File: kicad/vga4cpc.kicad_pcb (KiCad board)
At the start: 2 copper layers, 61.4 x 76.7 mm, 39 parts, among them J1 VGA socket, J2 CPC video port, SW1 VFreq sw, SW2 reset, U1 Pico

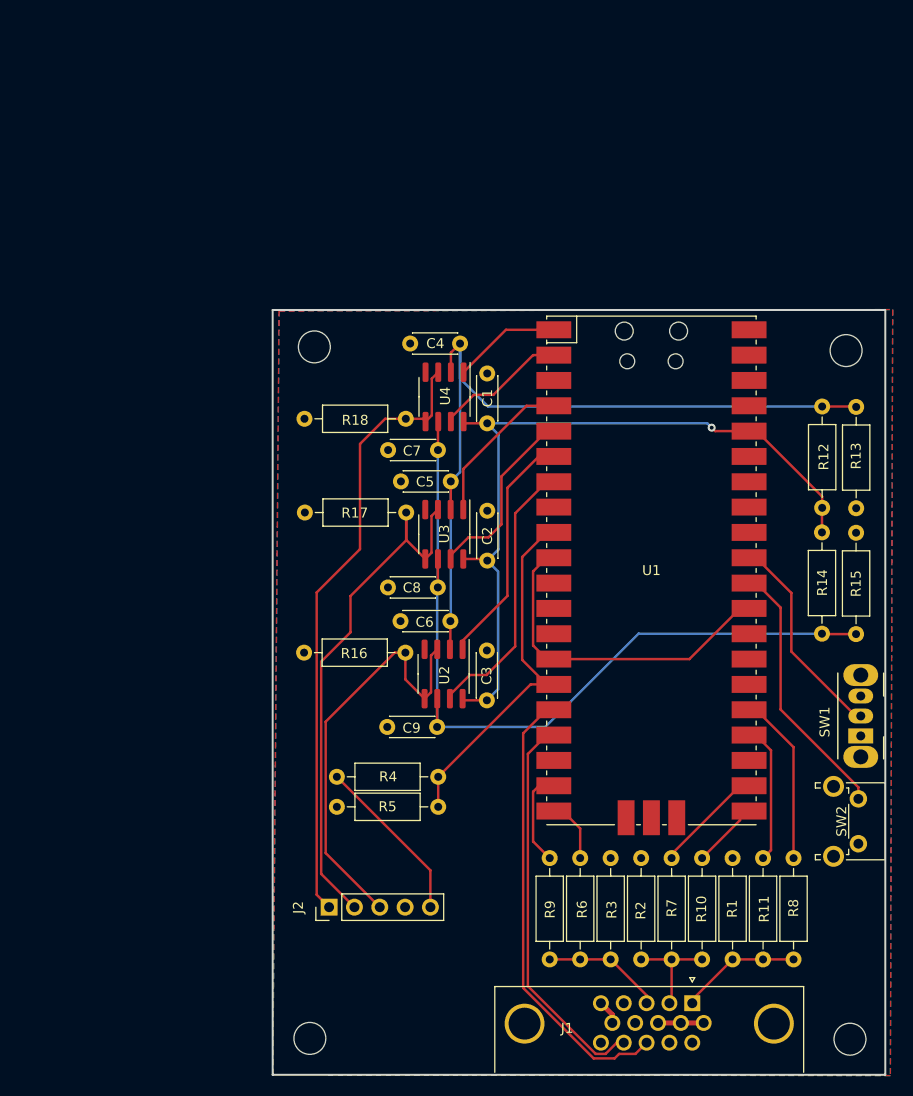
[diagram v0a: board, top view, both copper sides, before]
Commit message: Refactored
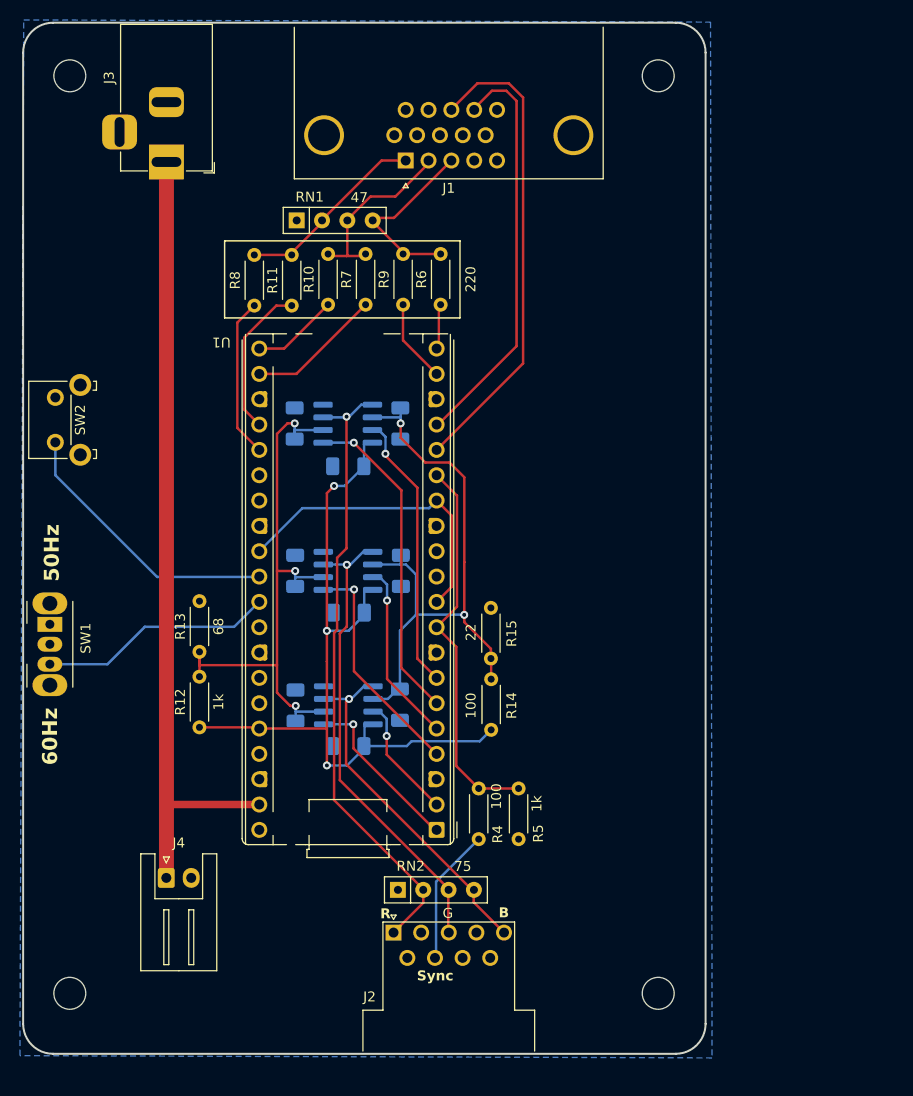
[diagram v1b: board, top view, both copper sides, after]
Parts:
- removed R1, R2, R3: 47, Resistor_THT:R_Axial_DIN0207_L6.3mm_D2.5mm_P10.16mm_Horizontal
- removed R16, R17, R18: 75, Resistor_THT:R_Axial_DIN0207_L6.3mm_D2.5mm_P10.16mm_Horizontal
- added J3: Barrel_Jack, Connector_BarrelJack:BarrelJack_Horizontal, F.Cu at (59.7, 36.6)
- added J4: Conn_01x02_Pin, Connector_JST:JST_XH_S2B-XH-A_1x02_P2.50mm_Horizontal, F.Cu at (59.7, 108.4)
- added RN1: 47, Resistor_THT:R_Array_SIP4, F.Cu at (72.8, 42.5)
- added RN2: 75, Resistor_THT:R_Array_SIP4, F.Cu at (82.9, 109.6)
- C1, C2, C3, C4, C5, C6, C7, C8, C9: footprint Capacitor_THT:C_Disc_D4.3mm_W1.9mm_P5.00mm -> Capacitor_SMD:C_1206_3216Metric_Pad1.33x1.80mm_HandSolder; moved to B.Cu
- J1: footprint Connector_Dsub:DSUB-15-HD_Female_Horizontal_P2.29x1.98mm_EdgePinOffset3.03mm_Housed_MountingHolesOffset4.94mm -> Connector_Dsub:DSUB-15-HD_Socket_Horizontal_P2.29x2.54mm_EdgePinOffset8.35mm_Housed_MountingHolesOffset10.89mm
- J2: value CPC video port -> DE9_Pins; footprint Connector_PinHeader_2.54mm:PinHeader_1x05_P2.54mm_Vertical -> Connector_Dsub:DSUB-9_Pins_Horizontal_P2.77x2.54mm_EdgePinOffset9.40mm
- R10, R11, R12, R13, R14, R4, R5, R6, R7, R8, R9: footprint Resistor_THT:R_Axial_DIN0207_L6.3mm_D2.5mm_P10.16mm_Horizontal -> Resistor_THT:R_Axial_DIN0204_L3.6mm_D1.6mm_P5.08mm_Horizontal
- R15: value 15 -> 22; footprint Resistor_THT:R_Axial_DIN0207_L6.3mm_D2.5mm_P10.16mm_Horizontal -> Resistor_THT:R_Axial_DIN0204_L3.6mm_D1.6mm_P5.08mm_Horizontal
- SW1: footprint Button_Switch_THT:SW_CuK_OS102011MA1QN1_SPDT_Angled -> Button_Switch_THT:SW_Slide_SPDT_Angled_CK_OS102011MA1Q
- SW2: footprint Button_Switch_THT:SW_Tactile_SPST_Angled_PTS645Vx31-2LFS -> Button_Switch_THT:SW_Tactile_SKHH_Angled
- U1: footprint pico:RPi_Pico_SMD_TH -> Pico:RaspberryPi_Pico_Common_THT_b
- U2, U3, U4: moved to B.Cu
- moved H1 102.6 mm to (109.0, 28.0), turned to 180 degrees
- moved J1 89.2 mm to (83.7, 36.5), turned to 180 degrees
- moved SW2 88.1 mm to (48.5, 64.8), turned to 90 degrees
- moved H2 82.6 mm to (50.0, 28.0), turned to 180 degrees
- moved SW1 82.1 mm to (48.0, 83.0), turned to -90 degrees
- moved R8 77.4 mm to (68.5, 51.0), turned to 90 degrees
- moved R11 72.8 mm to (72.2, 51.0), turned to 90 degrees
- moved R13 70.3 mm to (63.0, 85.8), turned to 90 degrees
- moved H3 69.3 mm to (50.0, 120.0), turned to 180 degrees
- moved R10 67.0 mm to (75.9, 50.9), turned to 90 degrees
- moved R12 66.2 mm to (63.0, 93.3)
- moved R7 63.4 mm to (79.7, 50.9), turned to 90 degrees
- moved R9 57.4 mm to (83.4, 50.9), turned to 90 degrees
- moved R6 57.2 mm to (87.2, 50.9), turned to 90 degrees
- moved C4 39.9 mm to (72.6, 91.2), turned to 90 degrees
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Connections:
- net 200mV renamed /Comparators/200mV
- net 430mV renamed /Comparators/600mV
- J2 pad 1: /Comparators/CPC_B -> /Comparators/CPC_R
- J2 pad 2: /Comparators/CPC_G -> GND
- J2 pad 3: /Comparators/CPC_R -> /Comparators/CPC_G
- J2 pad 5: /Connectors/CPC_CSYNC -> /Comparators/CPC_B
- SW1 pad 2: Net-(SW1-B) -> GND
- SW1 pad 3: GND -> Net-(SW1-C)
- U1 pad 31: Net-(SW1-B) -> Net-(SW1-C)
- U1 pad 39: unconnected-(U1-VSYS-Pad39) -> +5V
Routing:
- net +5V: track 0.00 -> 81.2 mm
- net /Comparators/CPC_B: track 62.0 -> 35.7 mm, vias 0 -> 1
- net Net-(SW1-C): track 0.00 -> 23.6 mm
- net /Comparators/200mV: track 81.4 -> 59.0 mm, vias 0 -> 3
- net /Comparators/600mV: track 82.0 -> 61.1 mm, vias 0 -> 2
- net /Comparators/CPC_R: track 42.6 -> 62.7 mm, vias 0 -> 1
- net Net-(SW1-B): track 20.0 -> 0.00 mm
- net /Comparators/R0: track 22.5 -> 32.5 mm, vias 0 -> 1
- net /Comparators/CPC_G: track 55.4 -> 47.3 mm, vias 0 -> 1
- net /Connectors/VGA_G: track 10.3 -> 18.4 mm
- net /Connectors/VGA_R: track 11.8 -> 19.2 mm
- net GND: track 7.03 -> 0.00 mm
- net /Connectors/VGA_B: track 12.0 -> 19.0 mm
- net /Comparators/G0: track 16.7 -> 23.2 mm, vias 0 -> 1
- net /Comparators/B0: track 11.7 -> 17.1 mm, vias 0 -> 1
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- removed copper zone on F.Cu, net GND
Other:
- board size 61.4 x 76.7 mm -> 68.4 x 103.4 mm
- board text added: "50Hz"
- board text added: "60Hz"
- board text added: "B"
- board text added: "G"
- board text added: "R"
- board text added: "Sync"
